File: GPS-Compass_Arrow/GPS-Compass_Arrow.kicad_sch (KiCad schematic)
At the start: 73 parts, among them J2 FFC2B28-12-G, U1 OSK3056A-LR, U2 MAX7219, U3 74HC165

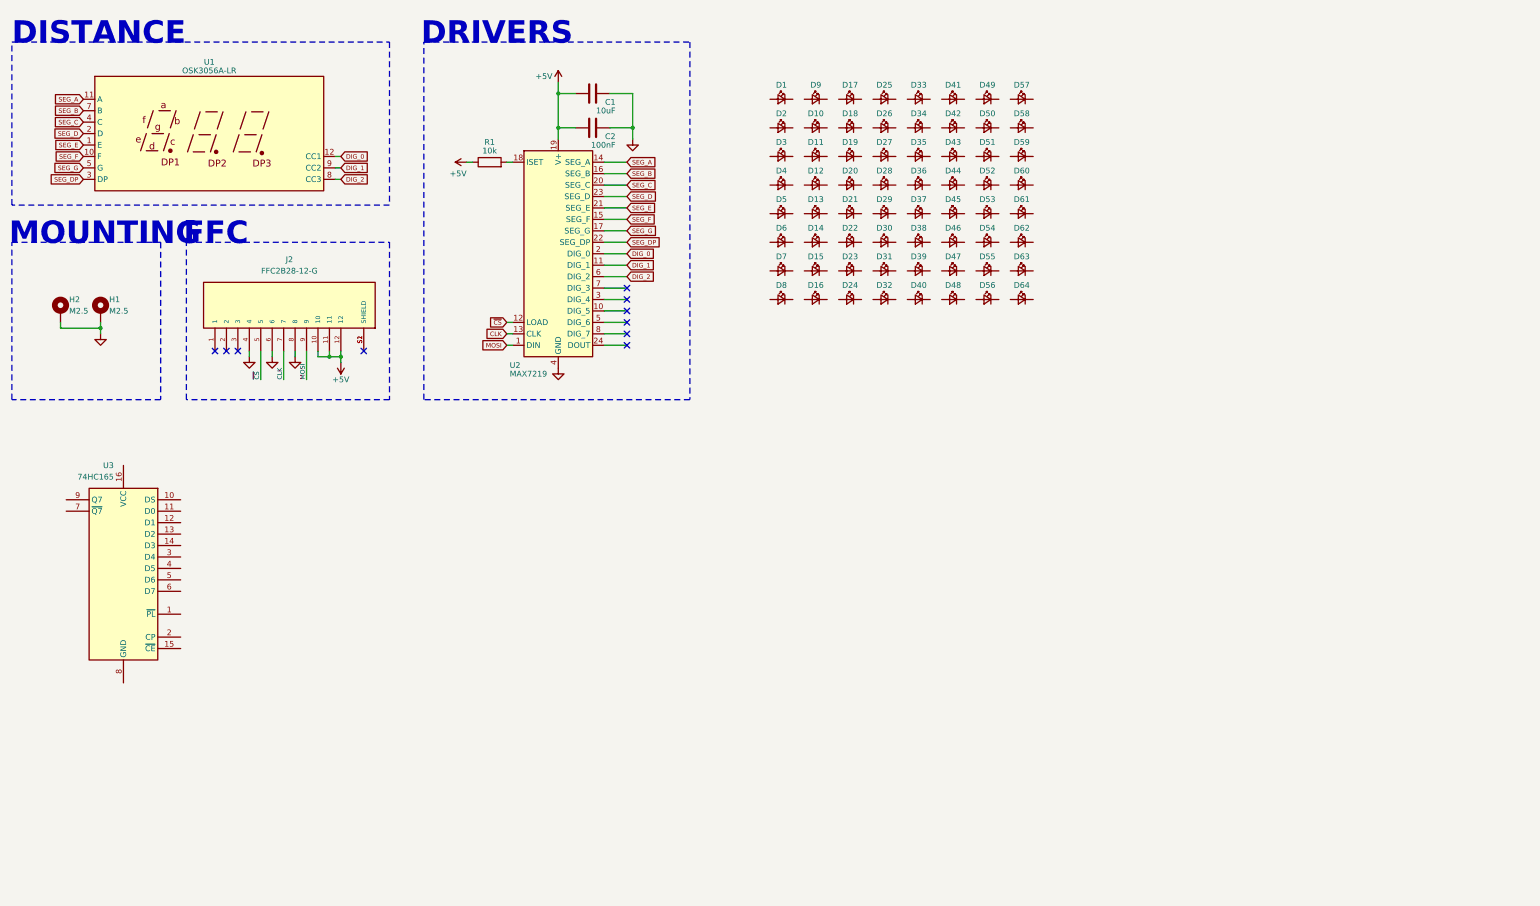
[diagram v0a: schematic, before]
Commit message: arrow pcb update
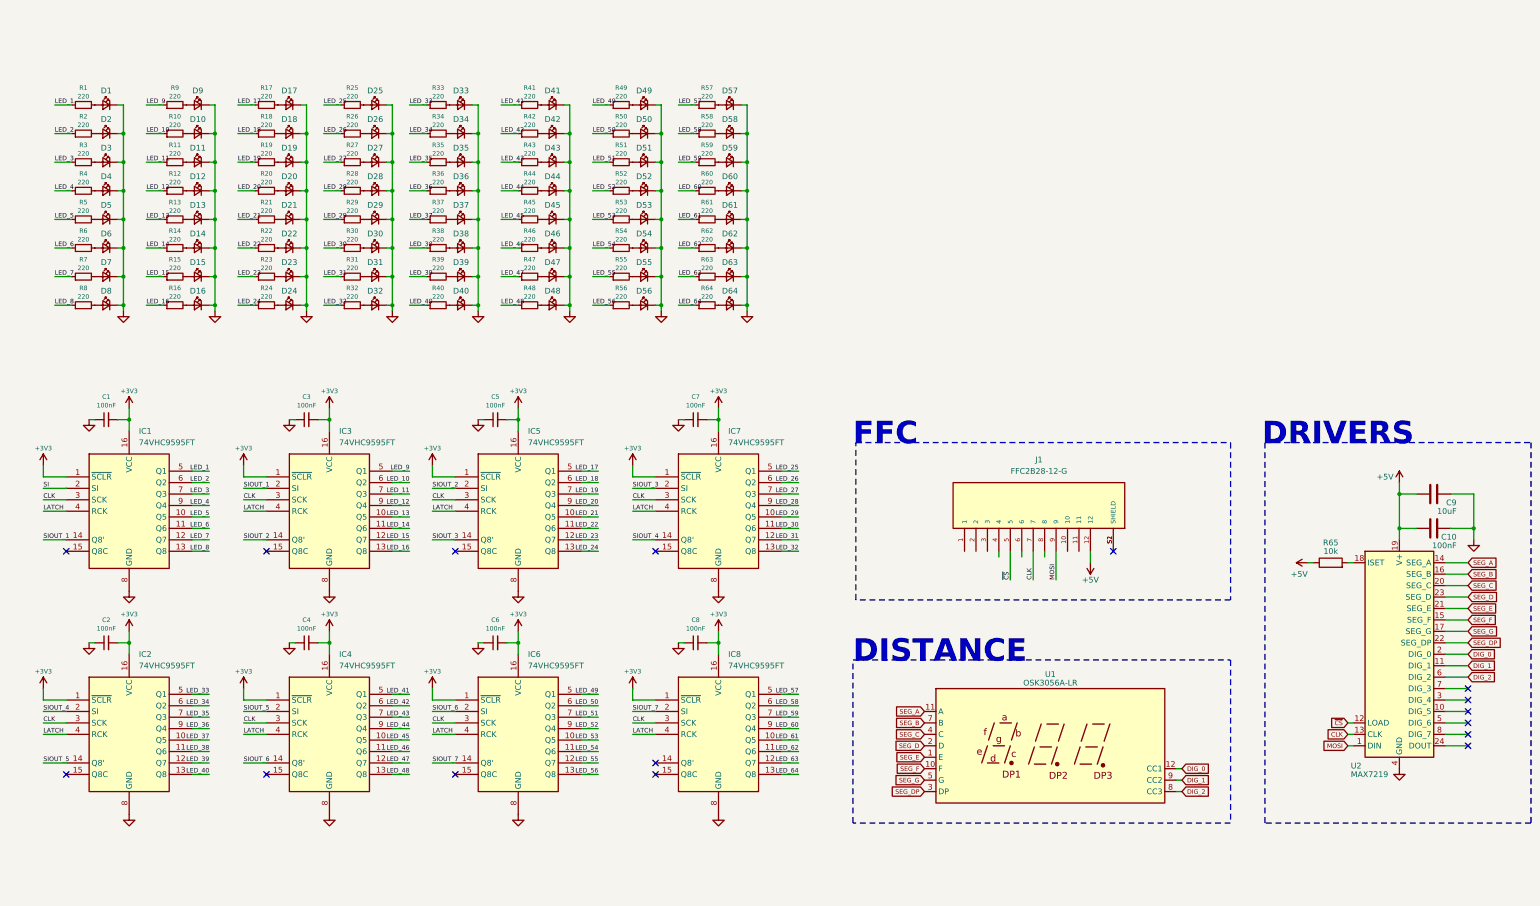
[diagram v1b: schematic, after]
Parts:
- removed H1, H2: M2.5, MountingHole:MountingHole_2.7mm_M2.5_Pad_Via, symbol Mechanical:MountingHole_Pad
- removed U3: 74HC165, symbol 74xx:74HC165
- added C1, C2, C3, C4, C5, C6, C7, C8: 100nF, Capacitor_SMD:C_0805_2012Metric, symbol Device:C_Small
- added IC1, IC2, IC3, IC4, IC5, IC6, IC7, IC8: 74VHC9595FT, gps-compass_brd:SOP65P640X120-16N, symbol gps-compass_sch:74VHC9595FT
- added R1, R10, R11, R12, R13, R14, R15, R16, R17, R18, R19, R2, R20, R21, R22, R23, R24, R25, R26, R27, R28, R29, R3, R30, R31, R32, R33, R34, R35, R36, R37, R38, R39, R4, R40, R41, R42, R43, R44, R45, R46, R47, R48, R49, R5, R50, R51, R52, R53, R54, R55, R56, R57, R58, R59, R6, R60, R61, R62, R63, R64, R7, R8, R9: 220, Resistor_SMD:R_0805_2012Metric, symbol Device:R_Small
- renumbered C2 to C10, C1 to C9, J2 to J1, R1 to R65
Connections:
- net +5V: no longer J1.10, J1.11
- net CLK: now also IC1.3 (SCK), IC2.3 (SCK), IC3.3 (SCK), IC4.3 (SCK), IC5.3 (SCK), IC6.3 (SCK), IC7.3 (SCK), IC8.3 (SCK)
- net GND: now also D1.1 (K), D10.1 (K), D11.1 (K), D12.1 (K), D13.1 (K), D14.1 (K), D15.1 (K), D16.1 (K), D17.1 (K), D18.1 (K), D19.1 (K), D2.1 (K), D20.1 (K), D21.1 (K), D22.1 (K), D23.1 (K), D24.1 (K), D25.1 (K), D26.1 (K), D27.1 (K), D28.1 (K), D29.1 (K), D3.1 (K), D30.1 (K), D31.1 (K), D32.1 (K), D33.1 (K), D34.1 (K), D35.1 (K), D36.1 (K), D37.1 (K), D38.1 (K), D39.1 (K), D4.1 (K), D40.1 (K), D41.1 (K), D42.1 (K), D43.1 (K), D44.1 (K), D45.1 (K), D46.1 (K), D47.1 (K), D48.1 (K), D49.1 (K), D5.1 (K), D50.1 (K), D51.1 (K), D52.1 (K), D53.1 (K), D54.1 (K), D55.1 (K), D56.1 (K), D57.1 (K), D58.1 (K), D59.1 (K), D6.1 (K), D60.1 (K), D61.1 (K), D62.1 (K), D63.1 (K), D64.1 (K), D7.1 (K), D8.1 (K), D9.1 (K), C1.1, C2.1, C3.1, C4.1, C5.1, C6.1, C7.1, C8.1, IC1.8 (GND), IC2.8 (GND), IC3.8 (GND), IC4.8 (GND), IC5.8 (GND), IC6.8 (GND), IC7.8 (GND), IC8.8 (GND); no longer J1.4, J1.6, J1.8
- net at D44.2 (A): now also R44.2
- net at D41.2 (A): now also R41.2
- net at D58.2 (A): now also R58.2
- net at D6.2 (A): now also R6.2
- net at D62.2 (A): now also R62.2
- net at D16.2 (A): now also R16.2
- net at D33.2 (A): now also R33.2
- net at D50.2 (A): now also R50.2
- net at D45.2 (A): now also R45.2
- net at D43.2 (A): now also R43.2
- net at D56.2 (A): now also R56.2
- net at D39.2 (A): now also R39.2
- net at D22.2 (A): now also R22.2
- net at D42.2 (A): now also R42.2
- net at D31.2 (A): now also R31.2
- net at D1.2 (A): now also R1.2
- net at D23.2 (A): now also R23.2
- net at D47.2 (A): now also R47.2
- net at D2.2 (A): now also R2.2
- net at D48.2 (A): now also R48.2
- net at D36.2 (A): now also R36.2
- net at D60.2 (A): now also R60.2
- net at D13.2 (A): now also R13.2
- net at D64.2 (A): now also R64.2
- net at D4.2 (A): now also R4.2
- net at D11.2 (A): now also R11.2
- net at D32.2 (A): now also R32.2
- net at D54.2 (A): now also R54.2
- net at D34.2 (A): now also R34.2
- net at D38.2 (A): now also R38.2
- net at D5.2 (A): now also R5.2
- net at D40.2 (A): now also R40.2
- net at D59.2 (A): now also R59.2
- net at D15.2 (A): now also R15.2
- net at D30.2 (A): now also R30.2
- net at D35.2 (A): now also R35.2
- net at D14.2 (A): now also R14.2
- net at D61.2 (A): now also R61.2
- net at D27.2 (A): now also R27.2
- net at D18.2 (A): now also R18.2
- net at D10.2 (A): now also R10.2
- net at D7.2 (A): now also R7.2
- net at D20.2 (A): now also R20.2
- net at D46.2 (A): now also R46.2
- net at D28.2 (A): now also R28.2
- net at D55.2 (A): now also R55.2
- net at D25.2 (A): now also R25.2
- net at D19.2 (A): now also R19.2
- net at D29.2 (A): now also R29.2
- net at D9.2 (A): now also R9.2
- net at D8.2 (A): now also R8.2
- net at D21.2 (A): now also R21.2
- net at D49.2 (A): now also R49.2
- net at D37.2 (A): now also R37.2
- net at D53.2 (A): now also R53.2
- net at D24.2 (A): now also R24.2
- net at D63.2 (A): now also R63.2
- net at D57.2 (A): now also R57.2
- net at D51.2 (A): now also R51.2
- net at D3.2 (A): now also R3.2
- net at D12.2 (A): now also R12.2
- net at D26.2 (A): now also R26.2
- net at D52.2 (A): now also R52.2
- net at D17.2 (A): now also R17.2
- new net +3V3: C1.2, C2.2, C3.2, C4.2, C5.2, C6.2, C7.2, C8.2, IC1.1 (~{SCLR}), IC1.16 (VCC), IC2.1 (~{SCLR}), IC2.16 (VCC), IC3.1 (~{SCLR}), IC3.16 (VCC), IC4.1 (~{SCLR}), IC4.16 (VCC), IC5.1 (~{SCLR}), IC5.16 (VCC), IC6.1 (~{SCLR}), IC6.16 (VCC), IC7.1 (~{SCLR}), IC7.16 (VCC), IC8.1 (~{SCLR}), IC8.16 (VCC)
- new net LATCH: IC1.4 (RCK), IC2.4 (RCK), IC3.4 (RCK), IC4.4 (RCK), IC5.4 (RCK), IC6.4 (RCK), IC7.4 (RCK), IC8.4 (RCK)
- new net LED_1: IC1.5 (Q1), R1.1
- new net LED_10: IC3.6 (Q2), R10.1
- new net LED_11: IC3.7 (Q3), R11.1
- new net LED_12: IC3.9 (Q4), R12.1
- new net LED_13: IC3.10 (Q5), R13.1
- new net LED_14: IC3.11 (Q6), R14.1
- new net LED_15: IC3.12 (Q7), R15.1
- new net LED_16: IC3.13 (Q8), R16.1
- new net LED_17: IC5.5 (Q1), R17.1
- new net LED_18: IC5.6 (Q2), R18.1
- new net LED_19: IC5.7 (Q3), R19.1
- new net LED_2: IC1.6 (Q2), R2.1
- new net LED_20: IC5.9 (Q4), R20.1
- new net LED_21: IC5.10 (Q5), R21.1
- new net LED_22: IC5.11 (Q6), R22.1
- new net LED_23: IC5.12 (Q7), R23.1
- new net LED_24: IC5.13 (Q8), R24.1
- new net LED_25: IC7.5 (Q1), R25.1
- new net LED_26: IC7.6 (Q2), R26.1
- new net LED_27: IC7.7 (Q3), R27.1
- new net LED_28: IC7.9 (Q4), R28.1
- new net LED_29: IC7.10 (Q5), R29.1
- new net LED_3: IC1.7 (Q3), R3.1
- new net LED_30: IC7.11 (Q6), R30.1
- new net LED_31: IC7.12 (Q7), R31.1
- new net LED_32: IC7.13 (Q8), R32.1
- new net LED_33: IC2.5 (Q1), R33.1
- new net LED_34: IC2.6 (Q2), R34.1
- new net LED_35: IC2.7 (Q3), R35.1
- new net LED_36: IC2.9 (Q4), R36.1
- new net LED_37: IC2.10 (Q5), R37.1
- new net LED_38: IC2.11 (Q6), R38.1
- new net LED_39: IC2.12 (Q7), R39.1
- new net LED_4: IC1.9 (Q4), R4.1
- new net LED_40: IC2.13 (Q8), R40.1
- new net LED_41: IC4.5 (Q1), R41.1
- new net LED_42: IC4.6 (Q2), R42.1
- new net LED_43: IC4.7 (Q3), R43.1
- new net LED_44: IC4.9 (Q4), R44.1
- new net LED_45: IC4.10 (Q5), R45.1
- new net LED_46: IC4.11 (Q6), R46.1
- new net LED_47: IC4.12 (Q7), R47.1
- new net LED_48: IC4.13 (Q8), R48.1
- new net LED_49: IC6.5 (Q1), R49.1
- new net LED_5: IC1.10 (Q5), R5.1
- new net LED_50: IC6.6 (Q2), R50.1
- new net LED_51: IC6.7 (Q3), R51.1
- new net LED_52: IC6.9 (Q4), R52.1
- new net LED_53: IC6.10 (Q5), R53.1
- new net LED_54: IC6.11 (Q6), R54.1
- new net LED_55: IC6.12 (Q7), R55.1
- new net LED_56: IC6.13 (Q8), R56.1
- new net LED_57: IC8.5 (Q1), R57.1
- new net LED_58: IC8.6 (Q2), R58.1
- new net LED_59: IC8.7 (Q3), R59.1
- new net LED_6: IC1.11 (Q6), R6.1
- new net LED_60: IC8.9 (Q4), R60.1
- new net LED_61: IC8.10 (Q5), R61.1
- new net LED_62: IC8.11 (Q6), R62.1
- new net LED_63: IC8.12 (Q7), R63.1
- new net LED_64: IC8.13 (Q8), R64.1
- new net LED_7: IC1.12 (Q7), R7.1
- new net LED_8: IC1.13 (Q8), R8.1
- new net LED_9: IC3.5 (Q1), R9.1
- new net SI: IC1.2 (SI)
- new net SIOUT_1: IC1.14 (Q8'), IC3.2 (SI)
- new net SIOUT_2: IC3.14 (Q8'), IC5.2 (SI)
- new net SIOUT_3: IC5.14 (Q8'), IC7.2 (SI)
- new net SIOUT_4: IC2.2 (SI), IC7.14 (Q8')
- new net SIOUT_5: IC2.14 (Q8'), IC4.2 (SI)
- new net SIOUT_6: IC4.14 (Q8'), IC6.2 (SI)
- new net SIOUT_7: IC6.14 (Q8'), IC8.2 (SI)
- no-connect marks 10 -> 16
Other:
- note removed: "MOUNTING"
- moved on the sheet: C10, C9, D1, D2, D3, D4, D5, D6, D7, D8, J1, R65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

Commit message: arrow pcb
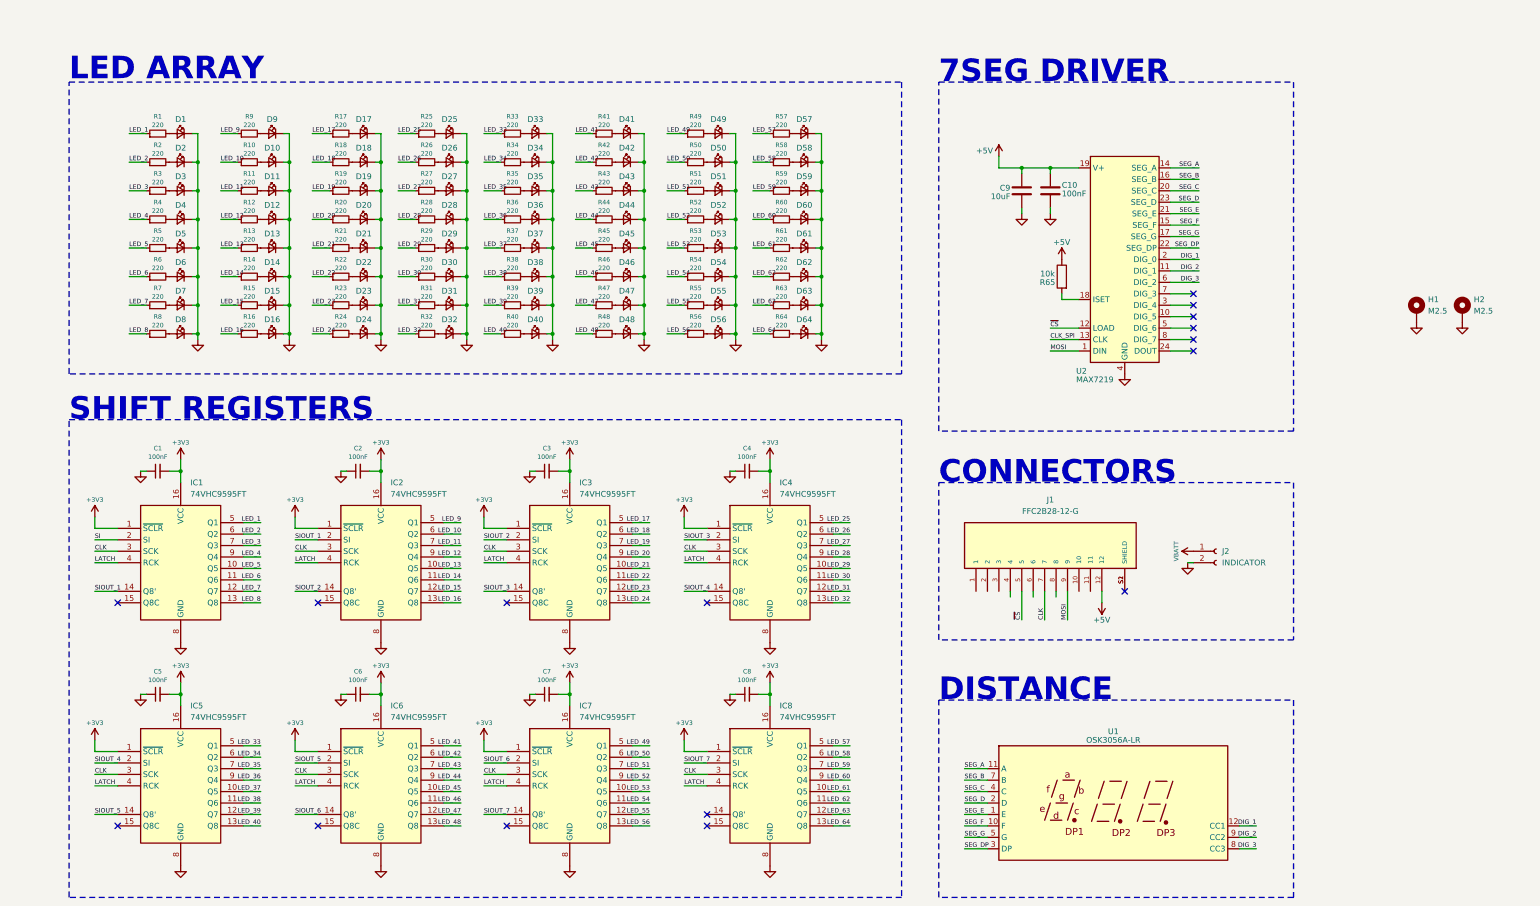
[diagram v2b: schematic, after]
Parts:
- added H1, H2: M2.5, MountingHole:MountingHole_2.5mm_Pad_Via, symbol Mechanical:MountingHole_Pad
- added J2: INDICATOR, Connector_PinHeader_2.54mm:PinHeader_1x02_P2.54mm_Vertical, symbol Connector:Conn_01x02_Socket
- R1, R10, R11, R12, R13, R14, R15, R16, R17, R18, R19, R2, R20, R21, R22, R23, R24, R25, R26, R27, R28, R29, R3, R30, R31, R32, R33, R34, R35, R36, R37, R38, R39, R4, R40, R41, R42, R43, R44, R45, R46, R47, R48, R49, R5, R50, R51, R52, R53, R54, R55, R56, R57, R58, R59, R6, R60, R61, R62, R63, R64, R7, R8, R9: footprint Resistor_SMD:R_0805_2012Metric -> Resistor_SMD:R_0603_1608Metric
- renumbered C3 to C2, C5 to C3, C7 to C4, C2 to C5, C4 to C6, C6 to C7, IC3 to IC2, IC5 to IC3, IC7 to IC4, IC2 to IC5, IC4 to IC6, IC6 to IC7
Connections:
- net DIG_0 is gone; now on net DIG_1: U1.12 (CC1), U2.2 (DIG_0)
- net +5V: now also C10.2, C9.2; no longer C10.1, C9.1
- net CLK: no longer U2.13 (CLK)
- net DIG_1: no longer U1.9 (CC2), U2.11 (DIG_1)
- net DIG_2: now also U1.9 (CC2), U2.11 (DIG_1); no longer U1.8 (CC3), U2.6 (DIG_2)
- net GND: now also C10.1, C9.1, H1.1, H2.1, J2.2 (Pin_2); no longer C10.2, C9.2
- new net CLK_SPI: U2.13 (CLK)
- new net DIG_3: U1.8 (CC3), U2.6 (DIG_2)
- new net VBATT: J2.1 (Pin_1)
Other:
- note added: "7SEG DRIVER"
- note added: "CONNECTORS"
- note added: "LED ARRAY"
- note added: "SHIFT REGISTERS"
- note removed: "DRIVERS"
- note removed: "FFC"
- moved on the sheet: C1, C10, C2, C3, C4, C5, C6, C7, C8, C9, D1, D10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
